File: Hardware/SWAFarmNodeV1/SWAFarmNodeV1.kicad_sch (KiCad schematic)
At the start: 27 parts, among them J1 DC_IN_12V, Q1 NMOS_30V_RDSon_20mOhm, U1 LT8610AC-3.3

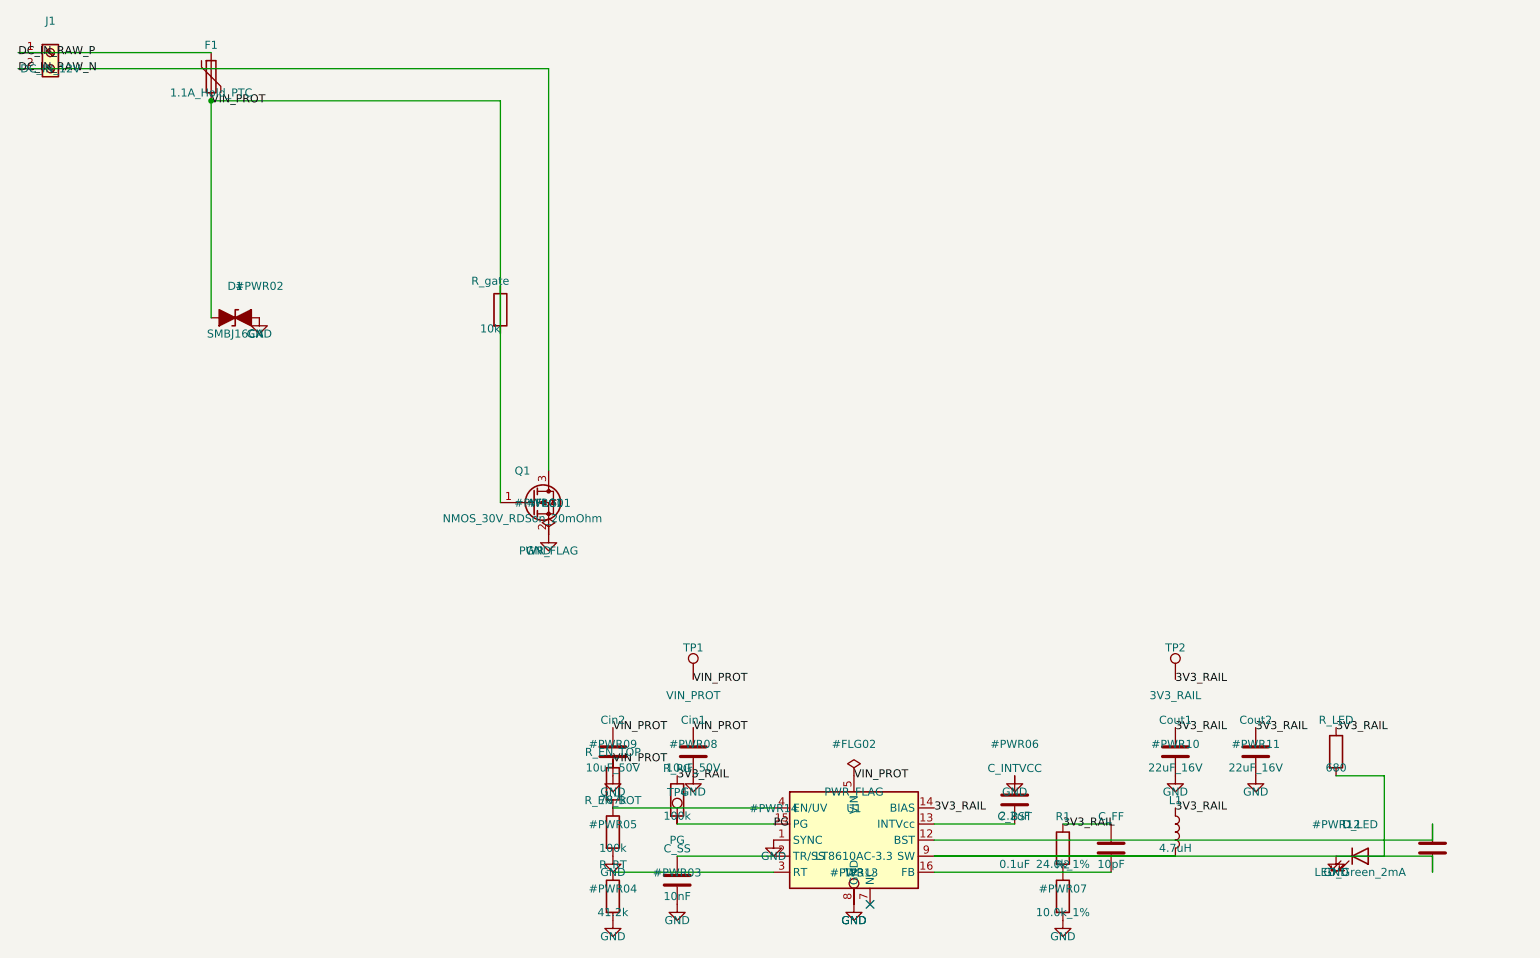
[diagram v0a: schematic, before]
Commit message: updated
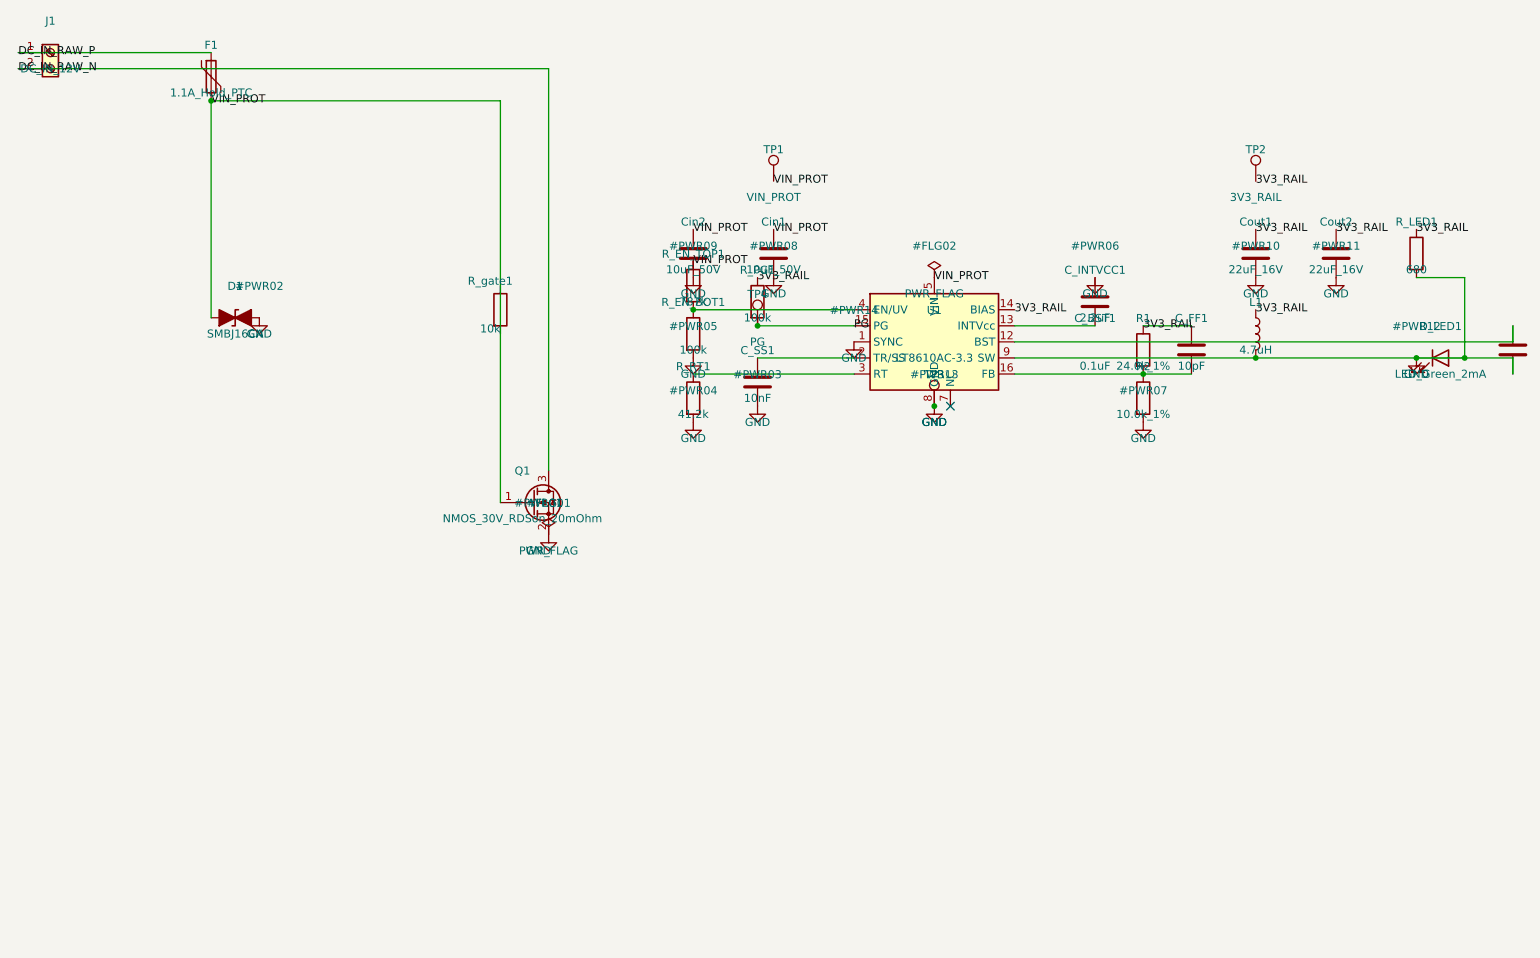
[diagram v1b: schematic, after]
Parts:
- renumbered C_BST to C_BST1, C_FF to C_FF1, C_INTVCC to C_INTVCC1, C_SS to C_SS1, D_LED to D_LED1, R_EN_BOT to R_EN_BOT1, R_EN_TOP to R_EN_TOP1, R_LED to R_LED1, R_PG to R_PG1, R_RT to R_RT1, R_gate to R_gate1
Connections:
- net GND: now also C_BST1.2, D_LED1.2 (A), L1.2, R_LED1.2, U1.10 (SW), U1.11 (SW), U1.9 (SW)
- net VIN_PROT: no longer R_gate1.1, R_gate1.2
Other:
- moved on the sheet: C_BST1, C_FF1, C_INTVCC1, C_SS1, Cin1, Cin2, Cout1, Cout2, D_LED1, L1, R1, R2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

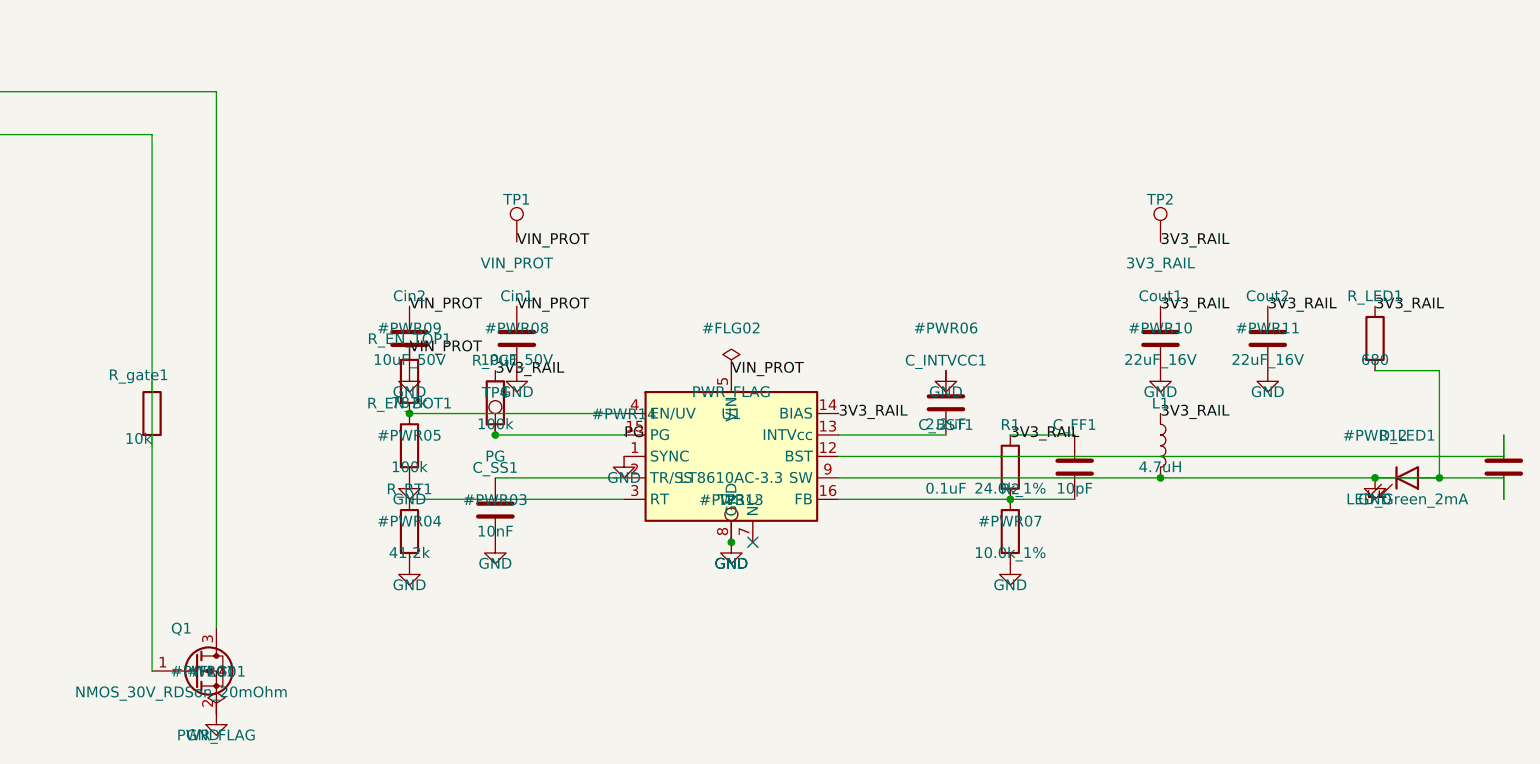
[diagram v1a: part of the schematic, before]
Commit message: updated
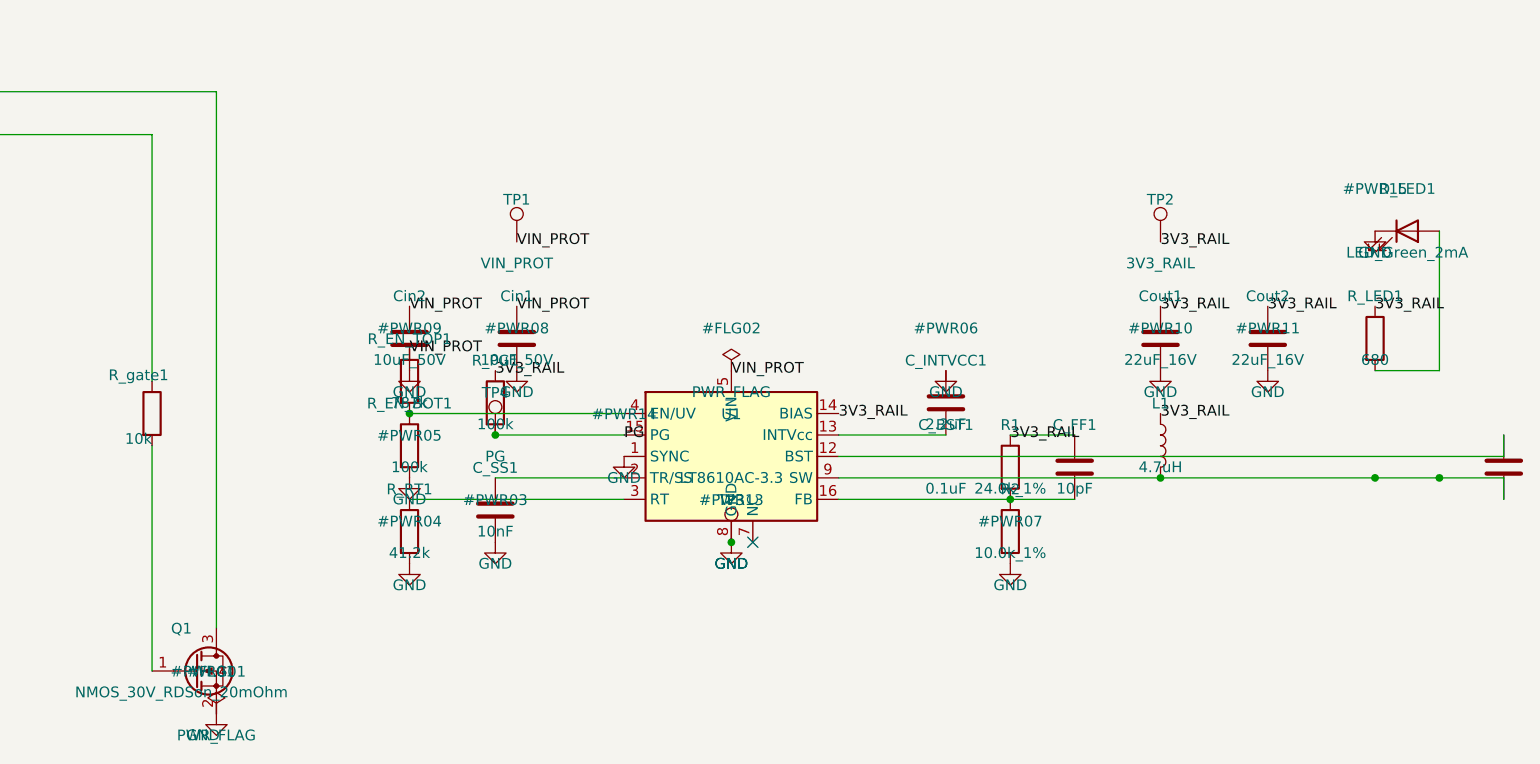
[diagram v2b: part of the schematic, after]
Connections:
- net GND: no longer C_BST1.2, D_LED1.2 (A), L1.2, R_LED1.2, U1.10 (SW), U1.11 (SW), U1.9 (SW)
- net VIN_PROT: now also R_gate1.1; no longer Q1.1 (G)
- net at R_gate1.2: now also Q1.1 (G)
- new net: C_BST1.2, L1.2, U1.10 (SW), U1.11 (SW), U1.9 (SW)
- new net: D_LED1.2 (A), R_LED1.2
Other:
- moved on the sheet: D_LED1
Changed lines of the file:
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@@
 	(wire
 		(pts
-			(xy 96.52 96.52) (xy 96.52 160.02)
+			(xy 96.52 96.52) (xy 96.52 125.73)
+		)
+		(stroke
+			(width 0)
+			(type default)
+		)
+	)
+	(wire
+		(pts
+			(xy 96.52 133.35) (xy 96.52 160.02)
 		)
 		(stroke
@@
 	(wire
 		(pts
-			(xy 248.92 124.46) (xy 248.92 137.16)
+			(xy 248.92 124.46) (xy 248.92 107.95)
 		)
 		(stroke
@@
 	)
 	(symbol
-		(lib_id "power:GND")
-		(at 241.3 137.16 0)
-		(unit 1)
-		(body_style 1)
-		(exclude_from_sim no)
-		(in_bom yes)
-		(on_board yes)
-		(in_pos_files yes)
-		(dnp no)
-		(property "Reference" "#PWR12"
-			(at 241.3 132.16 0)
-			(show_name no)
-			(do_not_autoplace no)
-			(effects
-				(font
-					(size 1.27 1.27)
-				)
-			)
-		)
-		(property "Value" "GND"
-			(at 241.3 139.7 0)
-			(show_name no)
-			(do_not_autoplace no)
-			(effects
-				(font
-					(size 1.27 1.27)
-				)
-			)
-		)
-		(property "Footprint" ""
-			(at 241.3 142.24 0)
-			(hide yes)
-			(show_name no)
-			(do_not_autoplace no)
-			(effects
-				(font
-					(size 1.27 1.27)
-				)
-			)
-		)
-		(property "Datasheet" ""
-			(at 241.3 137.16 0)
-			(show_name no)
-			(do_not_autoplace no)
-			(effects
-				(font
-					(size 1.27 1.27)
-				)
-			)
-		)
-		(property "Description" ""
-			(at 241.3 137.16 0)
-			(show_name no)
-			(do_not_autoplace no)
-			(effects
-				(font
-					(size 1.27 1.27)
-				)
-			)
-		)
-		(pin "1"
-		)
-		(instances
-			(project "SWAFarmNodeV1"
-				(path "/060522f3-d6eb-4e60-99ff-6cb93ab6e749"
-					(reference "#PWR12")
-					(unit 1)
-				)
-			)
-		)
-	)
-	(symbol
 		(lib_id "Device:R")
 		(at 241.3 120.65 0)
@@
 	(symbol
 		(lib_id "Device:LED")
-		(at 245.11 137.16 0)
+		(at 245.11 107.95 0)
 		(unit 1)
 		(body_style 1)
@@
 		(dnp no)
 		(property "Reference" "D_LED1"
-			(at 245.11 132.16 0)
+			(at 245.11 102.95 0)
 			(show_name no)
 			(do_not_autoplace no)
@@
 		)
 		(property "Value" "LED_Green_2mA"
-			(at 245.11 139.7 0)
+			(at 245.11 110.49 0)
 			(show_name no)
 			(do_not_autoplace no)
@@
 		)
 		(property "Footprint" "LED_SMD:LED_0805_2012Metric"
-			(at 245.11 142.24 0)
+			(at 245.11 113.03 0)
 			(hide yes)
 			(show_name no)
@@
 		)
 		(property "Datasheet" ""
-			(at 245.11 137.16 0)
+			(at 245.11 107.95 0)
 			(show_name no)
 			(do_not_autoplace no)
@@
 		)
 		(property "Description" ""
-			(at 245.11 137.16 0)
+			(at 245.11 107.95 0)
 			(show_name no)
 			(do_not_autoplace no)
@@
 					(unit 1)
 				)
+			)
+		)
+	)
+	(symbol
+		(lib_id "power:GND")
+		(at 241.3 107.95 0)
+		(unit 1)
+		(body_style 1)
+		(exclude_from_sim no)
+		(in_bom yes)
+		(on_board yes)
+		(in_pos_files yes)
+		(dnp no)
+		(property "Reference" "#PWR15"
+			(at 241.3 102.95 0)
+			(show_name no)
+			(do_not_autoplace no)
+			(effects
+				(font
+					(size 1.27 1.27)
+				)
+			)
+		)
+		(property "Value" "GND"
+			(at 241.3 110.49 0)
+			(show_name no)
+			(do_not_autoplace no)
+			(effects
+				(font
+					(size 1.27 1.27)
+				)
+			)
+		)
+		(property "Footprint" ""
+			(at 241.3 107.95 0)
+			(hide yes)
+			(show_name no)
+			(do_not_autoplace no)
+			(effects
+				(font
+					(size 1.27 1.27)
+				)
+			)
+		)
+		(property "Datasheet" ""
+			(at 241.3 107.95 0)
+			(show_name no)
+			(do_not_autoplace no)
+			(effects
+				(font
+					(size 1.27 1.27)
+				)
+			)
+		)
+		(property "Description" ""
+			(at 241.3 107.95 0)
+			(show_name no)
+			(do_not_autoplace no)
+			(effects
+				(font
+					(size 1.27 1.27)
+				)
+			)
+		)
+		(pin "1"
+		)
+		(instances
+			(project "SWAFarmNodeV1"
+				(path "/060522f3-d6eb-4e60-99ff-6cb93ab6e749"
+					(reference "#PWR15")
+					(unit 1)
+				)

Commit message: updated upto  step 9 - PCB Floor Planning & Component Placement
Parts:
- added C_BATSENSE1, C_BTN1, C_BTST1, C_BTST2, C_LORA_VDD1, C_MCU_VBAT1, C_MCU_VDD1, C_MCU_VDD2, C_MCU_VDD3, C_MCU_VDDA2, C_MCU_VDDUSB1, C_NRST1, C_RS485_VCC1, C_VC1_1, C_VC2_1, C_VC3_1: 100nF, Capacitor_SMD:C_0603_1608Metric, symbol Device:C
- added C_CAP1_1, C_REGN1, C_REGOUT1: 1uF, Capacitor_SMD:C_0805_2012Metric, symbol Device:C
- added C_LSE1, C_LSE2: 8pF, Capacitor_SMD:C_0603_1608Metric, symbol Device:C
- added C_MCU_BULK1, C_SOL_IN1: 4.7uF, Capacitor_SMD:C_0805_2012Metric, symbol Device:C
- added C_MCU_VDDA1: 1uF, Capacitor_SMD:C_0603_1608Metric, symbol Device:C
- added C_PMID1: 10uF, Capacitor_SMD:C_1210_3225Metric, symbol Device:C
- added C_RELAY_BULK1, C_SYS1: 22uF, Capacitor_SMD:C_1210_3225Metric, symbol Device:C
- added D2: SMBJ24A_class_unidirectional, Diode_SMD:D_SMB, symbol Device:D_TVS_Filled
- added D_ACT1: LED_Yellow_activity, LED_SMD:LED_0805_2012Metric, symbol Device:LED
- added D_CHG_STAT1: LED_Yellow_charge_status, LED_SMD:LED_0805_2012Metric, symbol Device:LED
- added D_RELAY1_FLYBACK1, D_RELAY2_FLYBACK1, D_RELAY3_FLYBACK1, D_RELAY4_FLYBACK1, D_RELAY5_FLYBACK1: S1M_1A_1000V_SMA, Diode_SMD:D_SMA, symbol Device:D
- added D_RELAY1_STATUS1, D_RELAY2_STATUS1, D_RELAY3_STATUS1, D_RELAY4_STATUS1, D_RELAY5_STATUS1: LED_Green_relay_status, LED_SMD:LED_0805_2012Metric, symbol Device:LED
- added D_RS485_TVS_A1, D_RS485_TVS_B1: SMBJ_class_RS485, Diode_SMD:D_SMB, symbol Device:D_TVS_Filled
- added D_SENSOR_PWR_TVS1: SMBJ18A_class_unidirectional, Diode_SMD:D_SMB, symbol Device:D_TVS_Filled
- added D_STATUS1: LED_Green_status, LED_SMD:LED_0805_2012Metric, symbol Device:LED
- added F2: 0.75A_Hold_PTC, Fuse:Fuse_1812_4532Metric, symbol Device:Polyfuse
- added F3: 10A_series_onetime, Fuse:Fuse_1206_3216Metric, symbol Device:Fuse
- added FB_MCU1: BLM18 class, Inductor_SMD:L_0603_1608Metric, symbol Device:FerriteBead
- added FB_RELAY_PWR1: Power Ferrite, 1A class, Inductor_SMD:L_1206_3216Metric, symbol Device:FerriteBead
- added F_RS485_A1, F_RS485_A2, F_RS485_A3, F_RS485_A4, F_RS485_A5, F_RS485_B1, F_RS485_B2, F_RS485_B3, F_RS485_B4, F_RS485_B5, F_RS485_PWR1, F_RS485_PWR2, F_RS485_PWR3, F_RS485_PWR4, F_RS485_PWR5: 0.2A_Hold_PTC, Fuse:Fuse_1206_3216Metric, symbol Device:Polyfuse
- added J2: SOLAR_IN_12V_class, TerminalBlock_Phoenix:TerminalBlock_Phoenix_MKDS-3-2-5.08_1x02_P5.08mm_Horizontal, symbol Connector:Screw_Terminal_01x02
- added J3: 4S_LiFePO4_Pack, TerminalBlock_Phoenix:TerminalBlock_Phoenix_MKDS-3-2-5.08_1x02_P5.08mm_Horizontal, symbol Connector:Screw_Terminal_01x02
- added J_DBG_UART1: Debug_Console, Connector_PinHeader_2.54mm:PinHeader_1x03_P2.54mm_Vertical, symbol Connector_Generic:Conn_01x03
- added J_LORA_ANT1: U.FL_to_SMA_pigtail, Connector_Coaxial:U.FL_Hirose_U.FL-R-SMT-1_Vertical, symbol Connector:Conn_Coaxial
- added J_RELAY11: Relay1_COM_NO_NC, TerminalBlock_Phoenix:TerminalBlock_Phoenix_MKDS-1,5-3-5.08_1x03_P5.08mm_Horizontal, symbol Connector_Generic:Conn_01x03
- added J_RELAY21: Relay2_COM_NO_NC, TerminalBlock_Phoenix:TerminalBlock_Phoenix_MKDS-1,5-3-5.08_1x03_P5.08mm_Horizontal, symbol Connector_Generic:Conn_01x03
- added J_RELAY31: Relay3_COM_NO_NC, TerminalBlock_Phoenix:TerminalBlock_Phoenix_MKDS-1,5-3-5.08_1x03_P5.08mm_Horizontal, symbol Connector_Generic:Conn_01x03
- added J_RELAY41: Relay4_COM_NO_NC, TerminalBlock_Phoenix:TerminalBlock_Phoenix_MKDS-1,5-3-5.08_1x03_P5.08mm_Horizontal, symbol Connector_Generic:Conn_01x03
- added J_RELAY51: Relay5_COM_NO_NC, TerminalBlock_Phoenix:TerminalBlock_Phoenix_MKDS-1,5-3-5.08_1x03_P5.08mm_Horizontal, symbol Connector_Generic:Conn_01x03
- added J_RS485_SENSOR1: Sensor1_A_B_PWR_GND, TerminalBlock_Phoenix:TerminalBlock_Phoenix_MKDS-1,5-4-5.08_1x04_P5.08mm_Horizontal, symbol Connector_Generic:Conn_01x04
- added J_RS485_SENSOR2: Sensor2_A_B_PWR_GND, TerminalBlock_Phoenix:TerminalBlock_Phoenix_MKDS-1,5-4-5.08_1x04_P5.08mm_Horizontal, symbol Connector_Generic:Conn_01x04
- added J_RS485_SENSOR3: Sensor3_A_B_PWR_GND, TerminalBlock_Phoenix:TerminalBlock_Phoenix_MKDS-1,5-4-5.08_1x04_P5.08mm_Horizontal, symbol Connector_Generic:Conn_01x04
- added J_RS485_SENSOR4: Sensor4_A_B_PWR_GND, TerminalBlock_Phoenix:TerminalBlock_Phoenix_MKDS-1,5-4-5.08_1x04_P5.08mm_Horizontal, symbol Connector_Generic:Conn_01x04
- added J_RS485_SENSOR5: Sensor5_A_B_PWR_GND, TerminalBlock_Phoenix:TerminalBlock_Phoenix_MKDS-1,5-4-5.08_1x04_P5.08mm_Horizontal, symbol Connector_Generic:Conn_01x04
- added J_SWD1: SWD_ARM10, Connector_PinHeader_1.27mm:PinHeader_2x05_P1.27mm_Vertical, symbol Connector_Generic:Conn_02x05_Odd_Even
- added K_RELAY11, K_RELAY21, K_RELAY31, K_RELAY41, K_RELAY51: FINDER-40.51.9.012.0000_12VDC_SPDT_10A, Relay_THT:Relay_SPDT_Finder_40.51, symbol Relay:FINDER-40.51
- added L_CHG1: 2.2uH_5A_class, Inductor_SMD:L_10.4x10.4_H4.8, symbol Device:L
- added NTC_CHG1, NTC_PROT1: 10k_NTC_-20to60C_class, Resistor_SMD:R_0805_2012Metric, symbol Device:Thermistor_NTC
- added Q2, Q_AC1, Q_AC2, Q_CHG1, Q_DSG1: NMOS_30V_RDSon_20mOhm, Package_TO_SOT_SMD:TO-252-2, symbol Transistor_FET:Q_NMOS_GSD
- added Q_RELAY11, Q_RELAY21, Q_RELAY31, Q_RELAY41, Q_RELAY51: NMOS_30V_RDSon_100mOhm_SOT23, Package_TO_SOT_SMD:SOT-23, symbol Transistor_FET:Q_NMOS_GSD
- added R_ACT1, R_CHG_STAT1, R_RELAY1_STATUS1, R_RELAY2_STATUS1, R_RELAY3_STATUS1, R_RELAY4_STATUS1, R_RELAY5_STATUS1: 1k, Resistor_SMD:R_0805_2012Metric, symbol Device:R
- added R_BATSENSE_BOT1: 180k, Resistor_SMD:R_0805_2012Metric, symbol Device:R
- added R_BATSENSE_TOP1: 680k, Resistor_SMD:R_0805_2012Metric, symbol Device:R
- added R_BIAS_PD1, R_BIAS_PU1: 560, Resistor_SMD:R_0805_2012Metric, symbol Device:R
- added R_BOOT0_1, R_BTN1, R_LORA_BOOT1, R_LORA_RST1, R_NRST1, R_gate2: 10k, Resistor_SMD:R_0805_2012Metric, symbol Device:R
- added R_I2C_SCL_PU1, R_I2C_SDA_PU1: 4.7k, Resistor_SMD:R_0805_2012Metric, symbol Device:R
- added R_ILIM1: TBD_verify_datasheet_ILIM_formula, Resistor_SMD:R_0805_2012Metric, symbol Device:R
- added R_PROG1: TBD_verify_datasheet_for_1.6A_target, Resistor_SMD:R_0805_2012Metric, symbol Device:R
- added R_QON1: 100k, Resistor_SMD:R_0805_2012Metric, symbol Device:R
- added R_RELAY1_GATE1, R_RELAY2_GATE1, R_RELAY3_GATE1, R_RELAY4_GATE1, R_RELAY5_GATE1: 100, Resistor_SMD:R_0603_1608Metric, symbol Device:R
- added R_RELAY1_PD1, R_RELAY2_PD1, R_RELAY3_PD1, R_RELAY4_PD1, R_RELAY5_PD1: 10k, Resistor_SMD:R_0603_1608Metric, symbol Device:R
- added R_SENSE1: 5mOhm_1percent_2512, Resistor_SMD:R_2512_6332Metric, symbol Device:R
- added R_STATUS1: 330, Resistor_SMD:R_0805_2012Metric, symbol Device:R
- added R_TERM1: 120, Resistor_SMD:R_0805_2012Metric, symbol Device:R
- added R_VC1_1, R_VC2_1, R_VC3_1: 1k, Resistor_SMD:R_0603_1608Metric, symbol Device:R
- added SW_DIP1: TERM_BIAS_SELECT, Button_Switch_THT:SW_DIP_SPSTx03_Slide_9.78x9.8mm_W7.62mm_P2.54mm, symbol Switch:SW_DIP_x03
- added SW_RESET1: Reset_Button, Button_Switch_SMD:SW_SPST_TL3342, symbol Switch:SW_Push
- added SW_USER1: User_Button, Button_Switch_SMD:SW_SPST_TL3342, symbol Switch:SW_Push
- added TP_BAT1: BAT_P, TestPoint:TestPoint_THTPad_1.5x1.5mm_Drill0.7mm, symbol Connector:TestPoint
- added TP_BATSENSE1: BATSENSE_MID, TestPoint:TestPoint_THTPad_1.5x1.5mm_Drill0.7mm, symbol Connector:TestPoint
- added TP_BOOT0_1: BOOT0, TestPoint:TestPoint_THTPad_1.5x1.5mm_Drill0.7mm, symbol Connector:TestPoint
- added TP_ISENSE_HI1: SRP, TestPoint:TestPoint_THTPad_1.5x1.5mm_Drill0.7mm, symbol Connector:TestPoint
- added TP_ISENSE_LO1: SRN_GND, TestPoint:TestPoint_THTPad_1.5x1.5mm_Drill0.7mm, symbol Connector:TestPoint
- added TP_LORA_BOOT1: LORA_BOOT0, TestPoint:TestPoint_THTPad_1.5x1.5mm_Drill0.7mm, symbol Connector:TestPoint
- added TP_LORA_RESET1: LORA_RESET_N, TestPoint:TestPoint_THTPad_1.5x1.5mm_Drill0.7mm, symbol Connector:TestPoint
- added TP_LORA_RX1: LORA_RX, TestPoint:TestPoint_THTPad_1.5x1.5mm_Drill0.7mm, symbol Connector:TestPoint
- added TP_LORA_STATUS1: LORA_STATUS, TestPoint:TestPoint_THTPad_1.5x1.5mm_Drill0.7mm, symbol Connector:TestPoint
- added TP_LORA_SWCLK1: LORA_SWCLK, TestPoint:TestPoint_THTPad_1.5x1.5mm_Drill0.7mm, symbol Connector:TestPoint
- added TP_LORA_SWDIO1: LORA_SWDIO, TestPoint:TestPoint_THTPad_1.5x1.5mm_Drill0.7mm, symbol Connector:TestPoint
- added TP_LORA_TX1: LORA_TX, TestPoint:TestPoint_THTPad_1.5x1.5mm_Drill0.7mm, symbol Connector:TestPoint
- added TP_MCU_RX1: MCU_RX, TestPoint:TestPoint_THTPad_1.5x1.5mm_Drill0.7mm, symbol Connector:TestPoint
- added TP_MCU_TX1: MCU_TX, TestPoint:TestPoint_THTPad_1.5x1.5mm_Drill0.7mm, symbol Connector:TestPoint
- added TP_NRST1: NRST, TestPoint:TestPoint_THTPad_1.5x1.5mm_Drill0.7mm, symbol Connector:TestPoint
- added TP_RELAY1_CTRL1: RELAY1_CTRL, TestPoint:TestPoint_THTPad_1.5x1.5mm_Drill0.7mm, symbol Connector:TestPoint
- added TP_RELAY2_CTRL1: RELAY2_CTRL, TestPoint:TestPoint_THTPad_1.5x1.5mm_Drill0.7mm, symbol Connector:TestPoint
- added TP_RELAY3_CTRL1: RELAY3_CTRL, TestPoint:TestPoint_THTPad_1.5x1.5mm_Drill0.7mm, symbol Connector:TestPoint
- added TP_RELAY4_CTRL1: RELAY4_CTRL, TestPoint:TestPoint_THTPad_1.5x1.5mm_Drill0.7mm, symbol Connector:TestPoint
- added TP_RELAY5_CTRL1: RELAY5_CTRL, TestPoint:TestPoint_THTPad_1.5x1.5mm_Drill0.7mm, symbol Connector:TestPoint
- added TP_RELAY_GND1: GND, TestPoint:TestPoint_THTPad_1.5x1.5mm_Drill0.7mm, symbol Connector:TestPoint
- added TP_RELAY_PWR1: RELAY_PWR, TestPoint:TestPoint_THTPad_1.5x1.5mm_Drill0.7mm, symbol Connector:TestPoint
- added TP_RS485_A1: RS485_A, TestPoint:TestPoint_THTPad_1.5x1.5mm_Drill0.7mm, symbol Connector:TestPoint
- added TP_RS485_B1: RS485_B, TestPoint:TestPoint_THTPad_1.5x1.5mm_Drill0.7mm, symbol Connector:TestPoint
- added TP_RS485_DERE1: RS485_DE_RE, TestPoint:TestPoint_THTPad_1.5x1.5mm_Drill0.7mm, symbol Connector:TestPoint
- added TP_RS485_RX1: RS485_RX, TestPoint:TestPoint_THTPad_1.5x1.5mm_Drill0.7mm, symbol Connector:TestPoint
- added TP_RS485_TX1: RS485_TX, TestPoint:TestPoint_THTPad_1.5x1.5mm_Drill0.7mm, symbol Connector:TestPoint
- added TP_SOLAR1: SOL_PROT, TestPoint:TestPoint_THTPad_1.5x1.5mm_Drill0.7mm, symbol Connector:TestPoint
- added TP_USER_BTN1: USER_BTN, TestPoint:TestPoint_THTPad_1.5x1.5mm_Drill0.7mm, symbol Connector:TestPoint
- added U_CHG1: BQ25798_substitutes_BQ25792, Package_DFN_QFN:Texas_RQM0029A_VQFN-29_4x4mm_P0.4mm, symbol Battery_Management:BQ25798
- added U_LORA1: RAK3172-IN865, RF_Module:RAK3172, symbol RF_Module:RAK3172-xx-8-SM-xI
- added U_MCU1: STM32L462RETx, Package_QFP:LQFP-64_10x10mm_P0.5mm, symbol MCU_ST_STM32L4:STM32L462RETx
- added U_PROT1: BQ76920PW, Package_SO:TSSOP-20_4.4x6.5mm_P0.65mm, symbol Battery_Management:BQ76920PW
- added U_RS485_1: THVD1450D, Package_SO:SOIC-8_3.9x4.9mm_P1.27mm, symbol Interface_UART:THVD1450D
- added Y_LSE1: 32.768kHz, Crystal:Crystal_SMD_3215-2Pin_3.2x1.5mm, symbol Device:Crystal
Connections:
- net 3V3_RAIL: now also C_LORA_VDD1.1, C_MCU_BULK1.1, C_MCU_VBAT1.1, C_MCU_VDD1.1, C_MCU_VDD2.1, C_MCU_VDD3.1, C_MCU_VDDUSB1.1, C_RS485_VCC1.1, FB_MCU1.1, J_SWD1.1 (Pin_1), R_BIAS_PU1.2, R_BTN1.1, R_CHG_STAT1.1, R_I2C_SCL_PU1.1, R_I2C_SDA_PU1.1, R_LORA_RST1.1, R_NRST1.1, U_LORA1.24 (VDD), U_MCU1.1 (VBAT), U_MCU1.19 (VDD), U_MCU1.32 (VDD), U_MCU1.48 (VDDUSB), U_MCU1.64 (VDD), U_RS485_1.8 (VCC)
- net GND: now also C_BATSENSE1.2, C_BTN1.2, C_CAP1_1.2, C_LORA_VDD1.2, C_LSE1.2, C_LSE2.1, C_LSE2.2, C_MCU_BULK1.2, C_MCU_VBAT1.2, C_MCU_VDD1.2, C_MCU_VDD2.2, C_MCU_VDD3.2, C_MCU_VDDA1.1, C_MCU_VDDA1.2, C_MCU_VDDA2.1, C_MCU_VDDA2.2, C_MCU_VDDUSB1.2, C_NRST1.2, C_PMID1.2, C_REGN1.2, C_REGOUT1.2, C_RELAY_BULK1.2, C_RS485_VCC1.2, C_SOL_IN1.2, C_SYS1.2, C_VC1_1.2, C_VC2_1.2, C_VC3_1.2, D2.2 (A2), D_ACT1.1 (K), D_CHG_STAT1.1 (K), D_RELAY1_STATUS1.1 (K), D_RELAY2_STATUS1.1 (K), D_RELAY3_STATUS1.1 (K), D_RELAY4_STATUS1.1 (K), D_RELAY5_STATUS1.1 (K), D_RS485_TVS_A1.2 (A2), D_RS485_TVS_B1.2 (A2), D_SENSOR_PWR_TVS1.2 (A2), D_STATUS1.1 (K), FB_MCU1.2, J_DBG_UART1.1 (Pin_1), J_LORA_ANT1.2 (Ext), J_RS485_SENSOR1.4 (Pin_4), J_RS485_SENSOR2.4 (Pin_4), J_RS485_SENSOR3.4 (Pin_4), J_RS485_SENSOR4.4 (Pin_4), J_RS485_SENSOR5.4 (Pin_4), J_SWD1.3 (Pin_3), J_SWD1.5 (Pin_5), J_SWD1.9 (Pin_9), NTC_CHG1.2, NTC_PROT1.2, Q2.2 (S), Q_RELAY11.2 (S), Q_RELAY21.2 (S), Q_RELAY31.2 (S), Q_RELAY41.2 (S), Q_RELAY51.2 (S), R_BATSENSE_BOT1.2, R_BIAS_PD1.2, R_BOOT0_1.2, R_ILIM1.2, R_LORA_BOOT1.2, R_PROG1.2, R_QON1.2, R_RELAY1_PD1.2, R_RELAY2_PD1.2, R_RELAY3_PD1.2, R_RELAY4_PD1.2, R_RELAY5_PD1.2, R_SENSE1.2, SW_RESET1.2, SW_USER1.2, TP_ISENSE_LO1.1, TP_RELAY_GND1.1, U_CHG1.13 (~{CE}), U_CHG1.27 (GND), U_LORA1.11 (GND), U_LORA1.17 (GND), U_LORA1.18 (GND), U_LORA1.23 (GND), U_LORA1.28 (GND), U_MCU1.12 (VSSA), U_MCU1.13 (VDDA), U_MCU1.18 (VSS), U_MCU1.31 (VSS), U_MCU1.4 (PC15), U_MCU1.47 (VSS), U_MCU1.63 (VSS), U_PROT1.19 (SRN), U_PROT1.3 (VSS), U_RS485_1.5 (GND), Y_LSE1.2
- net VIN_PROT: now also Q_AC1.3 (D), U_CHG1.9 (VAC1); no longer U1.5 (VIN), U1.6 (VIN)
- new net: D_ACT1.2 (A), R_ACT1.2
- new net: R_BIAS_PD1.1, SW_DIP1.3
- new net: J_LORA_ANT1.1 (In), U_LORA1.12 (RF)
- new net: R_BIAS_PU1.1, SW_DIP1.2
- new net: R_TERM1.1, SW_DIP1.1
- new net ACTIVITY_LED: R_ACT1.1, U_MCU1.39 (PC8)
- new net BATSENSE_MID: C_BATSENSE1.1, R_BATSENSE_BOT1.1, R_BATSENSE_TOP1.2, TP_BATSENSE1.1, U_MCU1.27 (PB1)
- new net BAT_P: F3.2, R_BATSENSE_TOP1.1, TP_BAT1.1, U_CHG1.18 (BATP), U_CHG1.22 (BAT), U_CHG1.23 (BAT), U_PROT1.10 (BAT), U_PROT1.12 (VC5), U_PROT1.13 (VC4), U_PROT1.9 (REGSRC)
- new net BOOT0: R_BOOT0_1.1, TP_BOOT0_1.1, U_MCU1.60 (PH3)
- new net BTST1_NODE: C_BTST1.1, U_CHG1.4 (BTST1)
- new net BTST2_NODE: C_BTST2.1, U_CHG1.19 (BTST2)
- new net CAP1_NODE: C_CAP1_1.1, U_PROT1.7 (CAP1)
- new net CELL_N: J3.2 (Pin_2), Q_DSG1.3 (D), U_PROT1.17 (VC0)
- new net CELL_TAP1: R_VC1_1.1, U_PROT1.16 (VC1)
- new net CELL_TAP1_FILT: C_VC1_1.1, R_VC1_1.2
- new net CELL_TAP2: R_VC2_1.1, U_PROT1.15 (VC2)
- new net CELL_TAP2_FILT: C_VC2_1.1, R_VC2_1.2
- new net CELL_TAP3: R_VC3_1.1, U_PROT1.14 (VC3)
- new net CELL_TAP3_FILT: C_VC3_1.1, R_VC3_1.2
- new net CHG_ALERT_N: U_CHG1.21 (~{INT}), U_MCU1.24 (PC4)
- new net CHG_STAT: D_CHG_STAT1.2 (A), R_CHG_STAT1.2, U_CHG1.1 (STAT)
- new net CHG_VBUS_INT: C_BTST1.2, C_BTST2.2, Q_AC1.2 (S), Q_AC2.2 (S), U_CHG1.2 (VBUS), U_CHG1.3 (VBUS)
- new net FET_MID: Q_CHG1.2 (S), Q_DSG1.2 (S)
- new net J3_BAT_P_RAW: F3.1, J3.1 (Pin_1)
- new net LORA_BOOT0: R_LORA_BOOT1.1, TP_LORA_BOOT1.1, U_LORA1.21 (BOOT0)
- new net LORA_RESET_N: R_LORA_RST1.2, TP_LORA_RESET1.1, U_LORA1.22 (~{RST}), U_MCU1.14 (PA0)
- new net LORA_RX: TP_LORA_RX1.1, U_LORA1.4 (PB6/UART1_TX), U_MCU1.17 (PA3)
- new net LORA_STATUS: TP_LORA_STATUS1.1, U_LORA1.32 (PB3/PIN_A0), U_MCU1.15 (PA1)
- new net LORA_SWCLK: TP_LORA_SWCLK1.1, U_LORA1.8 (PA14/SWCLK)
- new net LORA_SWDIO: TP_LORA_SWDIO1.1, U_LORA1.7 (PA13/SWDIO)
- new net LORA_TX: TP_LORA_TX1.1, U_LORA1.5 (PB7/UART1_RX), U_MCU1.16 (PA2)
- new net MCU_RX: J_DBG_UART1.3 (Pin_3), TP_MCU_RX1.1, U_MCU1.43 (PA10)
- new net MCU_TX: J_DBG_UART1.2 (Pin_2), TP_MCU_TX1.1, U_MCU1.42 (PA9)
- new net NET_CHG_GATE: Q_CHG1.1 (G), U_PROT1.2 (CHG)
- new net NET_CHG_SW1: L_CHG1.1, U_CHG1.28 (SW1)
- new net NET_CHG_SW2: L_CHG1.2, U_CHG1.26 (SW2)
- new net NET_DSG_GATE: Q_DSG1.1 (G), U_PROT1.1 (DSG)
- new net NET_ILIM_HIZ: R_ILIM1.1, U_CHG1.17 (ILIM_HIZ)
- new net NET_PROG: R_PROG1.1, U_CHG1.20 (PROG)
- new net NET_Q2_GATE: Q2.1 (G), R_gate2.2
- new net NET_QAC1_GATE: Q_AC1.1 (G), U_CHG1.11 (ACDRV1)
- new net NET_QAC2_GATE: Q_AC2.1 (G), U_CHG1.10 (ACDRV2)
- new net NET_QON: R_QON1.1, U_CHG1.12 (~{QON})
- new net NRST: C_NRST1.1, J_SWD1.10 (Pin_10), R_NRST1.2, SW_RESET1.1, TP_NRST1.1, U_MCU1.7 (NRST)
- new net NTC_CHG_NODE: NTC_CHG1.1, U_CHG1.16 (TS)
- new net NTC_PROT_NODE: NTC_PROT1.1, U_PROT1.6 (TS1)
- new net OSC32_IN: C_LSE1.1, U_MCU1.3 (PC14), Y_LSE1.1
- new net PMID_NODE: C_PMID1.1, U_CHG1.29 (PMID)
- new net PROT_ALERT_N: U_MCU1.25 (PC5), U_PROT1.20 (ALERT)
- new net PWR_I2C_SCL: R_I2C_SCL_PU1.2, U_CHG1.14 (SCL), U_MCU1.61 (PB8), U_PROT1.5 (SCL)
- new net PWR_I2C_SDA: R_I2C_SDA_PU1.2, U_CHG1.15 (SDA), U_MCU1.62 (PB9), U_PROT1.4 (SDA)
- new net REGN_NODE: C_REGN1.1, U_CHG1.5 (REGN)
- new net REGOUT_NODE: C_REGOUT1.1, U_PROT1.8 (REGOUT)
- new net RELAY1_COIL_RTN: D_RELAY1_FLYBACK1.2 (A), K_RELAY11.A2, Q_RELAY11.3 (D)
- new net RELAY1_COM: J_RELAY11.1 (Pin_1), K_RELAY11.11
- new net RELAY1_CTRL: R_RELAY1_GATE1.1, R_RELAY1_STATUS1.1, TP_RELAY1_CTRL1.1, U_MCU1.33 (PB12)
- new net RELAY1_GATE: Q_RELAY11.1 (G), R_RELAY1_GATE1.2, R_RELAY1_PD1.1
- new net RELAY1_LED_A: D_RELAY1_STATUS1.2 (A), R_RELAY1_STATUS1.2
- new net RELAY1_NC: J_RELAY11.3 (Pin_3), K_RELAY11.12
- new net RELAY1_NO: J_RELAY11.2 (Pin_2), K_RELAY11.14
- new net RELAY2_COIL_RTN: D_RELAY2_FLYBACK1.2 (A), K_RELAY21.A2, Q_RELAY21.3 (D)
- new net RELAY2_COM: J_RELAY21.1 (Pin_1), K_RELAY21.11
- new net RELAY2_CTRL: R_RELAY2_GATE1.1, R_RELAY2_STATUS1.1, TP_RELAY2_CTRL1.1, U_MCU1.34 (PB13)
- new net RELAY2_GATE: Q_RELAY21.1 (G), R_RELAY2_GATE1.2, R_RELAY2_PD1.1
- new net RELAY2_LED_A: D_RELAY2_STATUS1.2 (A), R_RELAY2_STATUS1.2
- new net RELAY2_NC: J_RELAY21.3 (Pin_3), K_RELAY21.12
- new net RELAY2_NO: J_RELAY21.2 (Pin_2), K_RELAY21.14
- new net RELAY3_COIL_RTN: D_RELAY3_FLYBACK1.2 (A), K_RELAY31.A2, Q_RELAY31.3 (D)
- new net RELAY3_COM: J_RELAY31.1 (Pin_1), K_RELAY31.11
- new net RELAY3_CTRL: R_RELAY3_GATE1.1, R_RELAY3_STATUS1.1, TP_RELAY3_CTRL1.1, U_MCU1.35 (PB14)
- new net RELAY3_GATE: Q_RELAY31.1 (G), R_RELAY3_GATE1.2, R_RELAY3_PD1.1
- new net RELAY3_LED_A: D_RELAY3_STATUS1.2 (A), R_RELAY3_STATUS1.2
- new net RELAY3_NC: J_RELAY31.3 (Pin_3), K_RELAY31.12
- new net RELAY3_NO: J_RELAY31.2 (Pin_2), K_RELAY31.14
- new net RELAY4_COIL_RTN: D_RELAY4_FLYBACK1.2 (A), K_RELAY41.A2, Q_RELAY41.3 (D)
- new net RELAY4_COM: J_RELAY41.1 (Pin_1), K_RELAY41.11
- new net RELAY4_CTRL: R_RELAY4_GATE1.1, R_RELAY4_STATUS1.1, TP_RELAY4_CTRL1.1, U_MCU1.36 (PB15)
- new net RELAY4_GATE: Q_RELAY41.1 (G), R_RELAY4_GATE1.2, R_RELAY4_PD1.1
- new net RELAY4_LED_A: D_RELAY4_STATUS1.2 (A), R_RELAY4_STATUS1.2
- new net RELAY4_NC: J_RELAY41.3 (Pin_3), K_RELAY41.12
- new net RELAY4_NO: J_RELAY41.2 (Pin_2), K_RELAY41.14
- new net RELAY5_COIL_RTN: D_RELAY5_FLYBACK1.2 (A), K_RELAY51.A2, Q_RELAY51.3 (D)
- new net RELAY5_COM: J_RELAY51.1 (Pin_1), K_RELAY51.11
- new net RELAY5_CTRL: R_RELAY5_GATE1.1, R_RELAY5_STATUS1.1, TP_RELAY5_CTRL1.1, U_MCU1.50 (PA15)
- new net RELAY5_GATE: Q_RELAY51.1 (G), R_RELAY5_GATE1.2, R_RELAY5_PD1.1
- new net RELAY5_LED_A: D_RELAY5_STATUS1.2 (A), R_RELAY5_STATUS1.2
- new net RELAY5_NC: J_RELAY51.3 (Pin_3), K_RELAY51.12
- new net RELAY5_NO: J_RELAY51.2 (Pin_2), K_RELAY51.14
- new net RELAY_PWR: C_RELAY_BULK1.1, D_RELAY1_FLYBACK1.1 (K), D_RELAY2_FLYBACK1.1 (K), D_RELAY3_FLYBACK1.1 (K), D_RELAY4_FLYBACK1.1 (K), D_RELAY5_FLYBACK1.1 (K), FB_RELAY_PWR1.2, K_RELAY11.A1, K_RELAY21.A1, K_RELAY31.A1, K_RELAY41.A1, K_RELAY51.A1, TP_RELAY_PWR1.1
- new net RS485_A: D_RS485_TVS_A1.1 (A1), F_RS485_A1.1, F_RS485_A2.1, F_RS485_A3.1, F_RS485_A4.1, F_RS485_A5.1, R_TERM1.2, SW_DIP1.5, TP_RS485_A1.1, U_RS485_1.6 (A)
- new net RS485_A_RAW1: F_RS485_A1.2, J_RS485_SENSOR1.1 (Pin_1)
- new net RS485_A_RAW2: F_RS485_A2.2, J_RS485_SENSOR2.1 (Pin_1)
- new net RS485_A_RAW3: F_RS485_A3.2, J_RS485_SENSOR3.1 (Pin_1)
- new net RS485_A_RAW4: F_RS485_A4.2, J_RS485_SENSOR4.1 (Pin_1)
- new net RS485_A_RAW5: F_RS485_A5.2, J_RS485_SENSOR5.1 (Pin_1)
- new net RS485_B: D_RS485_TVS_B1.1 (A1), F_RS485_B1.1, F_RS485_B2.1, F_RS485_B3.1, F_RS485_B4.1, F_RS485_B5.1, SW_DIP1.4, SW_DIP1.6, TP_RS485_B1.1, U_RS485_1.7 (B)
- new net RS485_B_RAW1: F_RS485_B1.2, J_RS485_SENSOR1.2 (Pin_2)
- new net RS485_B_RAW2: F_RS485_B2.2, J_RS485_SENSOR2.2 (Pin_2)
- new net RS485_B_RAW3: F_RS485_B3.2, J_RS485_SENSOR3.2 (Pin_2)
- new net RS485_B_RAW4: F_RS485_B4.2, J_RS485_SENSOR4.2 (Pin_2)
- new net RS485_B_RAW5: F_RS485_B5.2, J_RS485_SENSOR5.2 (Pin_2)
- new net RS485_DE_RE: TP_RS485_DERE1.1, U_MCU1.28 (PB2), U_RS485_1.2 (~{RE}), U_RS485_1.3 (DE)
- new net RS485_RX: TP_RS485_RX1.1, U_MCU1.30 (PB11), U_RS485_1.1 (RO)
- new net RS485_TX: TP_RS485_TX1.1, U_MCU1.29 (PB10), U_RS485_1.4 (DI)
- new net SENSE_SRP: Q_CHG1.3 (D), R_SENSE1.1, TP_ISENSE_HI1.1, U_PROT1.18 (SRP)
- new net SOL_IN_RAW_N: J2.2 (Pin_2), Q2.3 (D)
- new net SOL_IN_RAW_P: F2.1, J2.1 (Pin_1)
- new net SOL_PROT: C_SOL_IN1.1, D2.1 (A1), F2.2, Q_AC2.3 (D), R_gate2.1, TP_SOLAR1.1, U_CHG1.8 (VAC2)
- new net STATUS_LED: D_STATUS1.2 (A), R_STATUS1.1, R_STATUS1.2, U_MCU1.2 (PC13)
- new net SWCLK: J_SWD1.4 (Pin_4), U_MCU1.49 (PA14)
- new net SWDIO: J_SWD1.2 (Pin_2), U_MCU1.46 (PA13)
- new net SWO: J_SWD1.6 (Pin_6), U_MCU1.55 (PB3)
- new net USER_BTN: C_BTN1.1, R_BTN1.2, SW_USER1.1, TP_USER_BTN1.1, U_MCU1.37 (PC6)
- new net VSYS: C_SYS1.1, U1.5 (VIN), U1.6 (VIN), U_CHG1.25 (SYS)
- new net VSYS_RAW_OUT: D_SENSOR_PWR_TVS1.1 (A1), FB_RELAY_PWR1.1, F_RS485_PWR1.1, F_RS485_PWR2.1, F_RS485_PWR3.1, F_RS485_PWR4.1, F_RS485_PWR5.1
- new net VSYS_RAW_OUT1: F_RS485_PWR1.2, J_RS485_SENSOR1.3 (Pin_3)
- new net VSYS_RAW_OUT2: F_RS485_PWR2.2, J_RS485_SENSOR2.3 (Pin_3)
- new net VSYS_RAW_OUT3: F_RS485_PWR3.2, J_RS485_SENSOR3.3 (Pin_3)
- new net VSYS_RAW_OUT4: F_RS485_PWR4.2, J_RS485_SENSOR4.3 (Pin_3)
- new net VSYS_RAW_OUT5: F_RS485_PWR5.2, J_RS485_SENSOR5.3 (Pin_3)
- no-connect marks 1 -> 3
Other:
- company: (none) -> SWAFarm
- title: (none) -> SWAFarm Node V1
